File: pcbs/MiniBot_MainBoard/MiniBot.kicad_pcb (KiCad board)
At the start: 4 copper layers, 21.2 x 28 mm, 60 parts, among them IC1 MMC5633NJL, IC2 MIC23050-SYML-TR, J1 Conn_01x08, J2 Conn_01x02, J3 GSB1C41110SSHR, U1 ESP32-C3-MINI-1-H4X, U3 MCP73832-2-OT, U4 STSPIN220, U5 STSPIN220

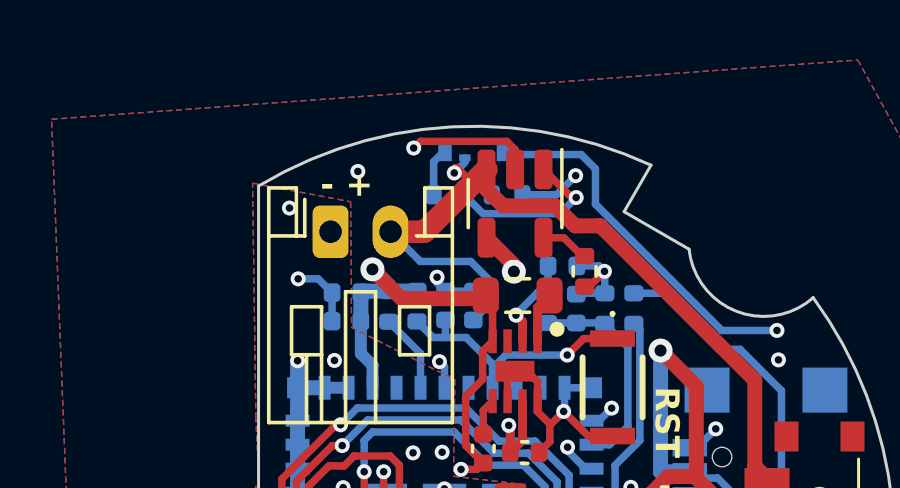
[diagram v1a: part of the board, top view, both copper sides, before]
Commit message: fix stupid bad led symbol, general improvements to minibot fw
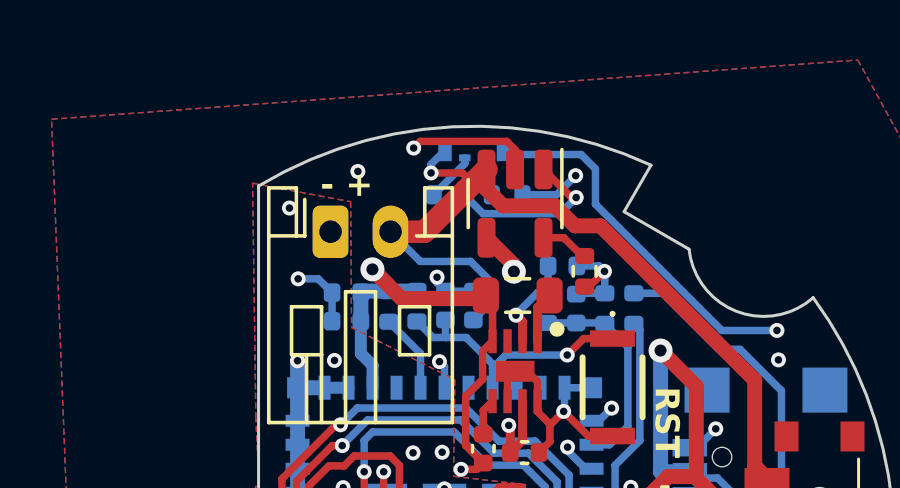
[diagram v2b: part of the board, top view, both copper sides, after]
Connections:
- LED1 pad 3: +BATT -> /LED_R
- LED1 pad 4: /LED_R -> +BATT
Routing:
- net +BATT: track 26.8 -> 27.8 mm
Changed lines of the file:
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@@
       (net 31 "Net-(LED1-T1-)") (pinfunction "T1-") (pintype "passive"))
     (pad "3" smd rect (at 0.315 -0.477 90) (size 0.23 0.38) (layers "B.Cu" "B.Paste" "B.Mask")
+      (net 73 "/LED_R") (pinfunction "R6-") (pintype "passive"))
+    (pad "4" smd rect (at 0.975 -0.227 180) (size 0.45 0.72) (layers "B.Cu" "B.Paste" "B.Mask")
       (net 30 "+BATT") (pinfunction "R6+") (pintype "passive"))
-    (pad "4" smd rect (at 0.975 -0.227 180) (size 0.45 0.72) (layers "B.Cu" "B.Paste" "B.Mask")
-      (net 73 "/LED_R") (pinfunction "R6-") (pintype "passive"))
   )
   (footprint "minibot:BGA4C40P2X2_85X85X60" (layer "B.Cu")
@@
   (segment (start 121.0575 87.0675) (end 121.2875 86.8375) (width 0.75) (layer "F.Cu") (net 30))
   (segment (start 130.69 96.265) (end 131.1 96.675) (width 0.5) (layer "F.Cu") (net 30))
-  (segment (start 120.698949 86.313202) (end 120.763202 86.313202) (width 0.25) (layer "F.Cu") (net 30))
+  (segment (start 119.9 86.490702) (end 120.940702 86.490702) (width 0.25) (layer "F.Cu") (net 30))
   (segment (start 130.69 93.399166) (end 130.69 96.265) (width 0.5) (layer "F.Cu") (net 30))
   (segment (start 121.2875 86.8375) (end 121.75 86.375) (width 0.75) (layer "F.Cu") (net 30))
-  (segment (start 120.763202 86.313202) (end 121.2875 86.8375) (width 0.25) (layer "F.Cu") (net 30))
+  (segment (start 120.940702 86.490702) (end 121.2875 86.8375) (width 0.25) (layer "F.Cu") (net 30))
   (segment (start 119.675 88.45) (end 121.0575 87.0675) (width 0.75) (layer "F.Cu") (net 30))
   (segment (start 125.545834 88.255) (end 130.69 93.399166) (width 0.5) (layer "F.Cu") (net 30))
-  (via (at 120.673949 86.490702) (size 0.5) (drill 0.25) (layers "F.Cu" "B.Cu") (net 30))
-  (segment (start 121.025 85.987) (end 121.025 86.139651) (width 0.25) (layer "B.Cu") (net 30))
-  (segment (start 121.025 86.139651) (end 120.673949 86.490702) (width 0.25) (layer "B.Cu") (net 30))
+  (via (at 119.9 86.490702) (size 0.5) (drill 0.25) (layers "F.Cu" "B.Cu") (net 30))
+  (segment (start 119.9 86.202) (end 120.365 85.737) (width 0.25) (layer "B.Cu") (net 30))
   (segment (start 119.54 89.44) (end 121.22078 89.44) (width 0.25) (layer "B.Cu") (net 30))
   (segment (start 121.22078 89.44) (end 121.895 90.11422) (width 0.25) (layer "B.Cu") (net 30))
   (segment (start 118.55 88.45) (end 119.54 89.44) (width 0.25) (layer "B.Cu") (net 30))
   (segment (start 121.895 90.11422) (end 121.895 90.805) (width 0.25) (layer "B.Cu") (net 30))
+  (segment (start 119.9 86.490702) (end 119.9 86.202) (width 0.25) (layer "B.Cu") (net 30))
   (segment (start 121.895 90.805) (end 121.31 91.39) (width 0.25) (layer "B.Cu") (net 30))
   (segment (start 121.655 85.987) (end 121.655 86.9475) (width 0.25) (layer "B.Cu") (net 31))
@@
   (segment (start 114.625 110.322978) (end 114.625 99.225) (width 0.25) (layer "In2.Cu") (net 72))
   (segment (start 115.707022 111.405) (end 114.625 110.322978) (width 0.25) (layer "In2.Cu") (net 72))
-  (segment (start 119.985 87.2175) (end 119.985 86.117) (width 0.25) (layer "B.Cu") (net 73))
-  (segment (start 119.985 86.117) (end 120.365 85.737) (width 0.25) (layer "B.Cu") (net 73))
+  (segment (start 119.985 87.2175) (end 121.025 86.1775) (width 0.25) (layer "B.Cu") (net 73))
+  (segment (start 121.025 86.1775) (end 121.025 85.987) (width 0.25) (layer "B.Cu") (net 73))
   (zone (net 0) (net_name "") (layers "F.Cu" "In1.Cu" "In2.Cu" "B.Cu") (hatch edge 0.5)
     (connect_pads (clearance 0))
